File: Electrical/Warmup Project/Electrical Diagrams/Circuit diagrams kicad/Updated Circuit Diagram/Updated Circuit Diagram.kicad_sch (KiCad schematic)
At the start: 26 parts, among them M1 Motor_DC, M2 Motor_DC, M3 Motor_DC, U3 MCP2562-H_SN, U4 Teensy4.1, U5 MCP2562-H_SN, U7 MCP2562-H_SN, U8 HX711, U9 HX711

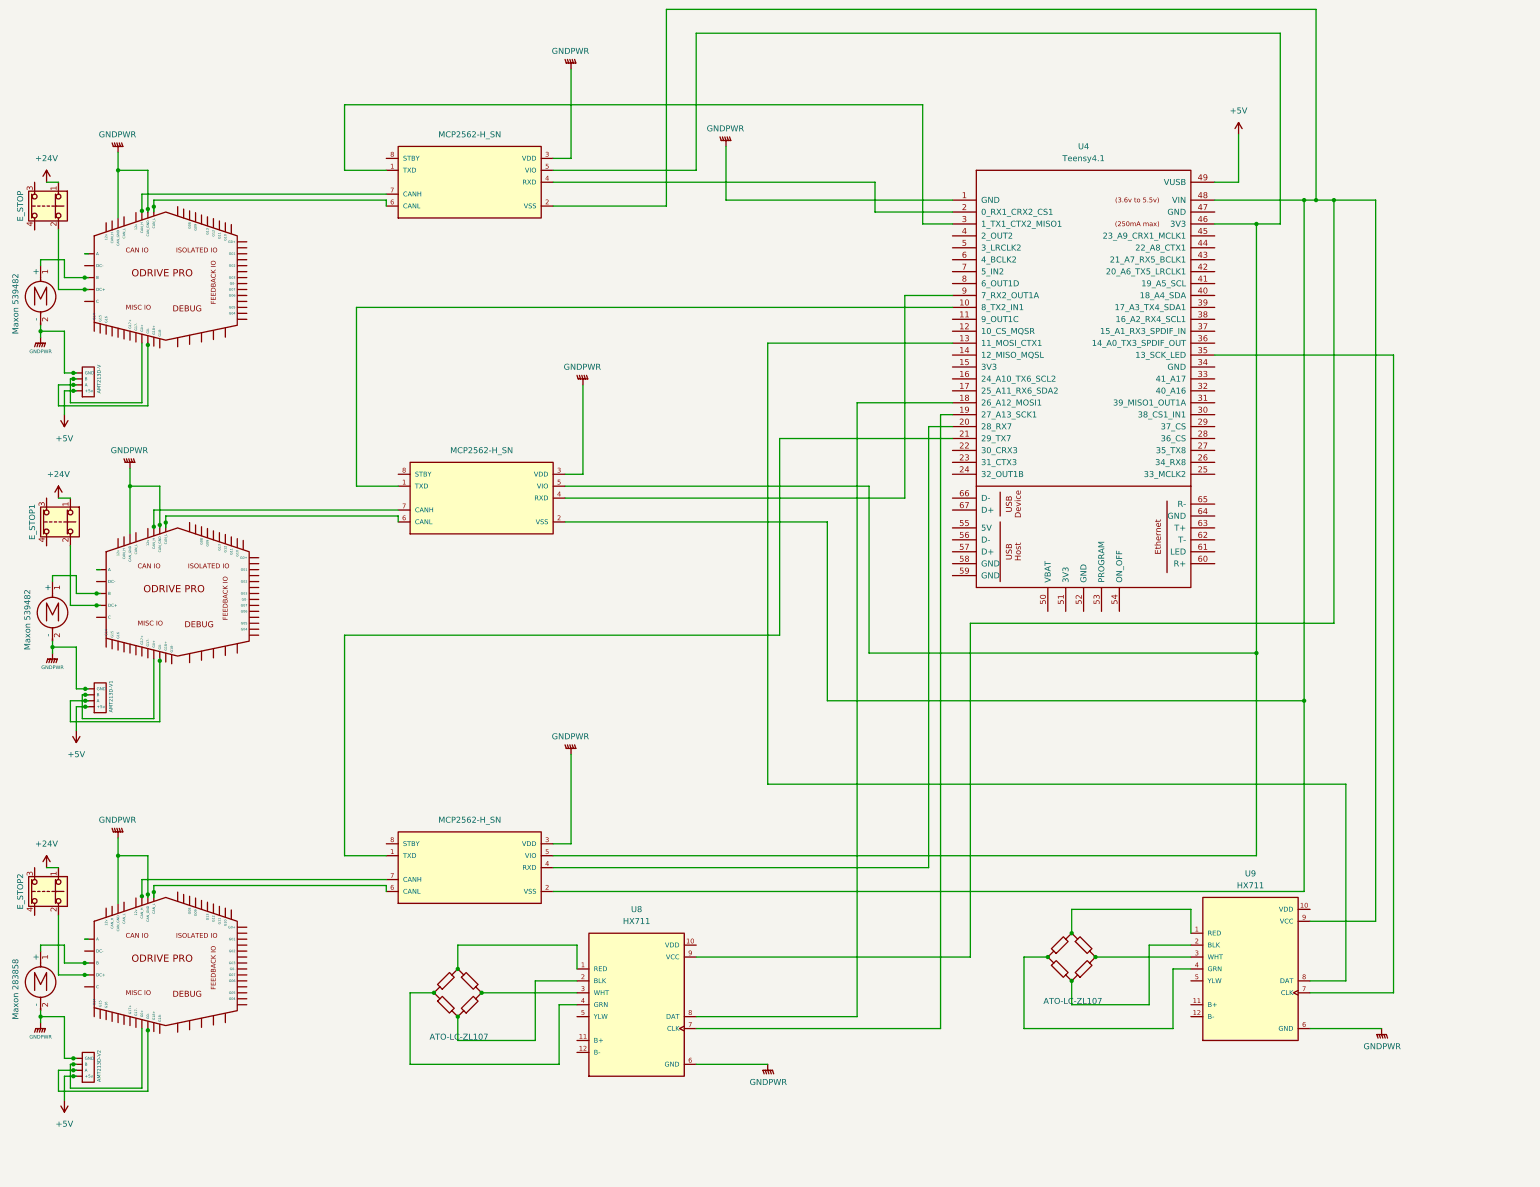
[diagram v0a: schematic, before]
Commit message: Hopefully working?
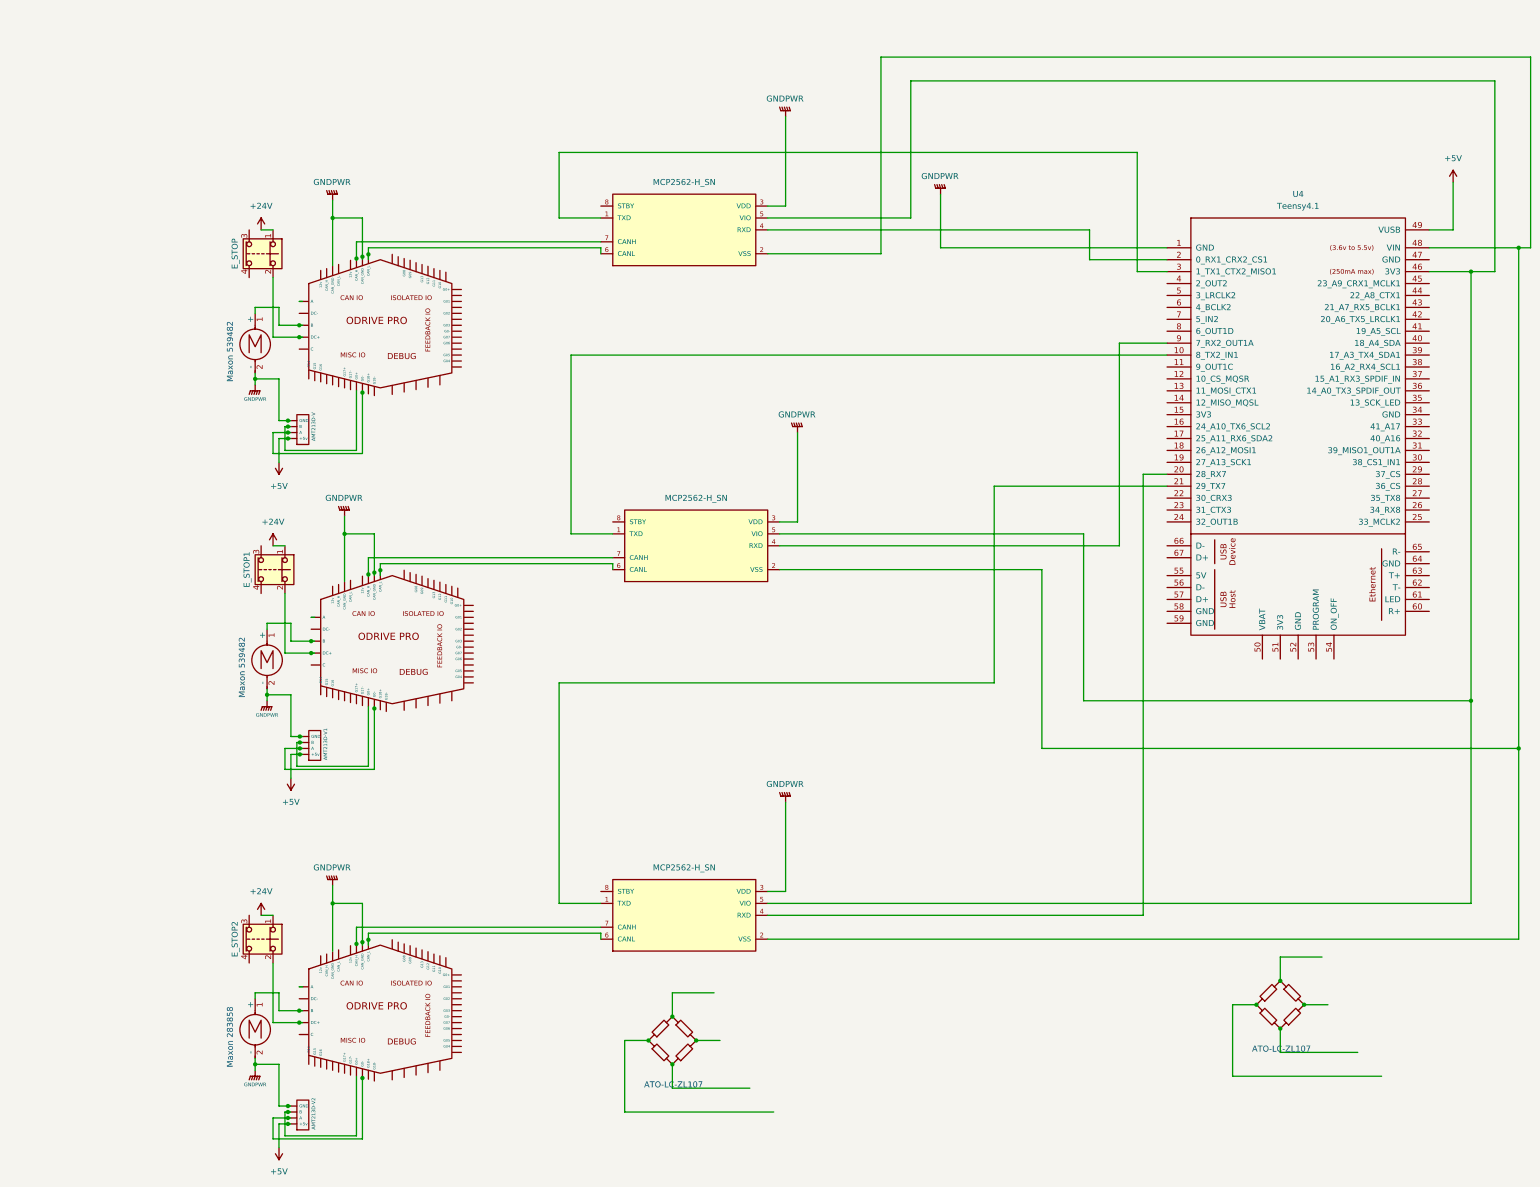
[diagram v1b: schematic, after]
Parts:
- removed R2, R3, R4, R5: R_45deg, symbol Device:R_45deg
- removed U8, U9: HX711, SEN-13879:SPARKFUN_SEN-13879, symbol SEN-13879:SEN-13879
- added R10, R11, R12, R9: R_45deg, symbol Device:R_45deg
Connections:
- new net: AMT213D-V2. (GND), U6. (x2)
- new net: R10.2, R12.1
- new net: R11.2, R12.2
- new net: R10.1, R9.1
- new net: R11.1, R9.2
- new net: AMT213D-V1. (GND), U2. (x2)
- new net: AMT213D-V. (GND), U1. (x2)
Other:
- moved on the sheet: AMT213D-V, AMT213D-V1, AMT213D-V2, E_STOP, E_STOP1, E_STOP2, U4
